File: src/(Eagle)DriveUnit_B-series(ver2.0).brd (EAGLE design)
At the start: 65.7 x 51 mm, 67 parts, among them IC1 A3921, SW1 TVAF06-A020B-R, SW2 TVAF06-A020B-R, SW3 THAF01-NC-R, SW4 SS-12D00G3

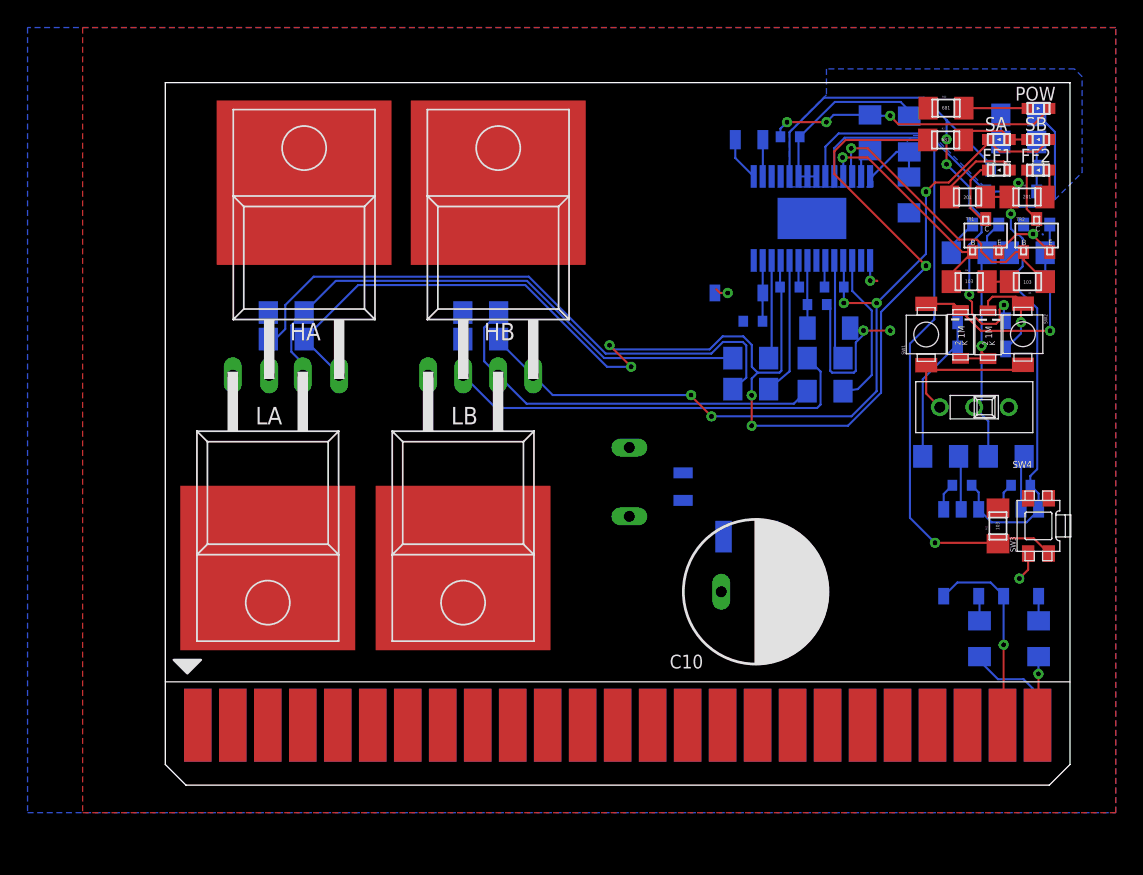
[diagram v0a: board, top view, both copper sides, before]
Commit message: 配線の終了
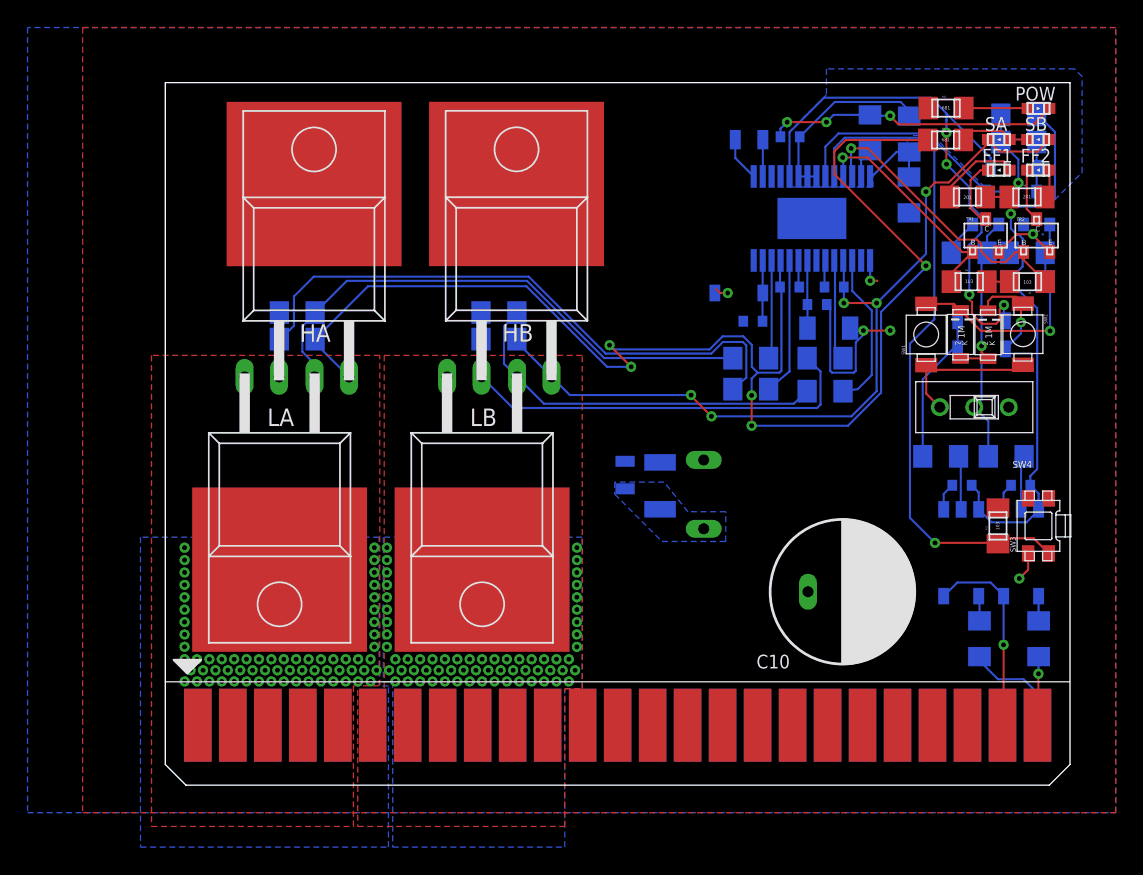
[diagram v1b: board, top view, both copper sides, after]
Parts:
- moved C12 7.31 mm to (35.9, 21.7), turned to 90 degrees
- moved C10 6.30 mm to (49.2, 14.0)
- moved C11 5.47 mm to (39.1, 21.1)
- moved C13 4.29 mm to (33.4, 22.5)
- moved LB 1.39 mm to (23.0, 24.6)
- moved HB 1.33 mm to (25.5, 34.7)
- moved R18 1.32 mm to (22.9, 34.3)
- moved R19 1.32 mm to (25.5, 32.4)
- moved LA 0.87 mm to (8.30, 24.6)
- moved R15 0.80 mm to (8.28, 34.3)
- moved R16 0.80 mm to (10.9, 32.4)
- moved HA 0.73 mm to (10.8, 34.7)
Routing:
- net V5: track 52.9 -> 56.0 mm
- net SB: track 63.5 -> 62.3 mm, vias 5 -> 69
- net N$21: track 33.4 -> 32.2 mm
- net N$26: track 29.2 -> 27.9 mm
- net SA: track 100.2 -> 99.4 mm, vias 5 -> 71
- net DIR: track 41.6 -> 42.3 mm
- net N$25: track 39.7 -> 39.0 mm
- net N$13: track 44.0 -> 43.4 mm
- added copper zone on layer 1, net SA
- added copper zone on layer 16, net SA
- added copper zone on layer 1, net SB
- added copper zone on layer 16, net SB
- added copper zone on layer 16, net VCC
